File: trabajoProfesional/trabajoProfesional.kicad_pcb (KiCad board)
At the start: 2 copper layers, 191.6 x 115.6 mm, 130 parts

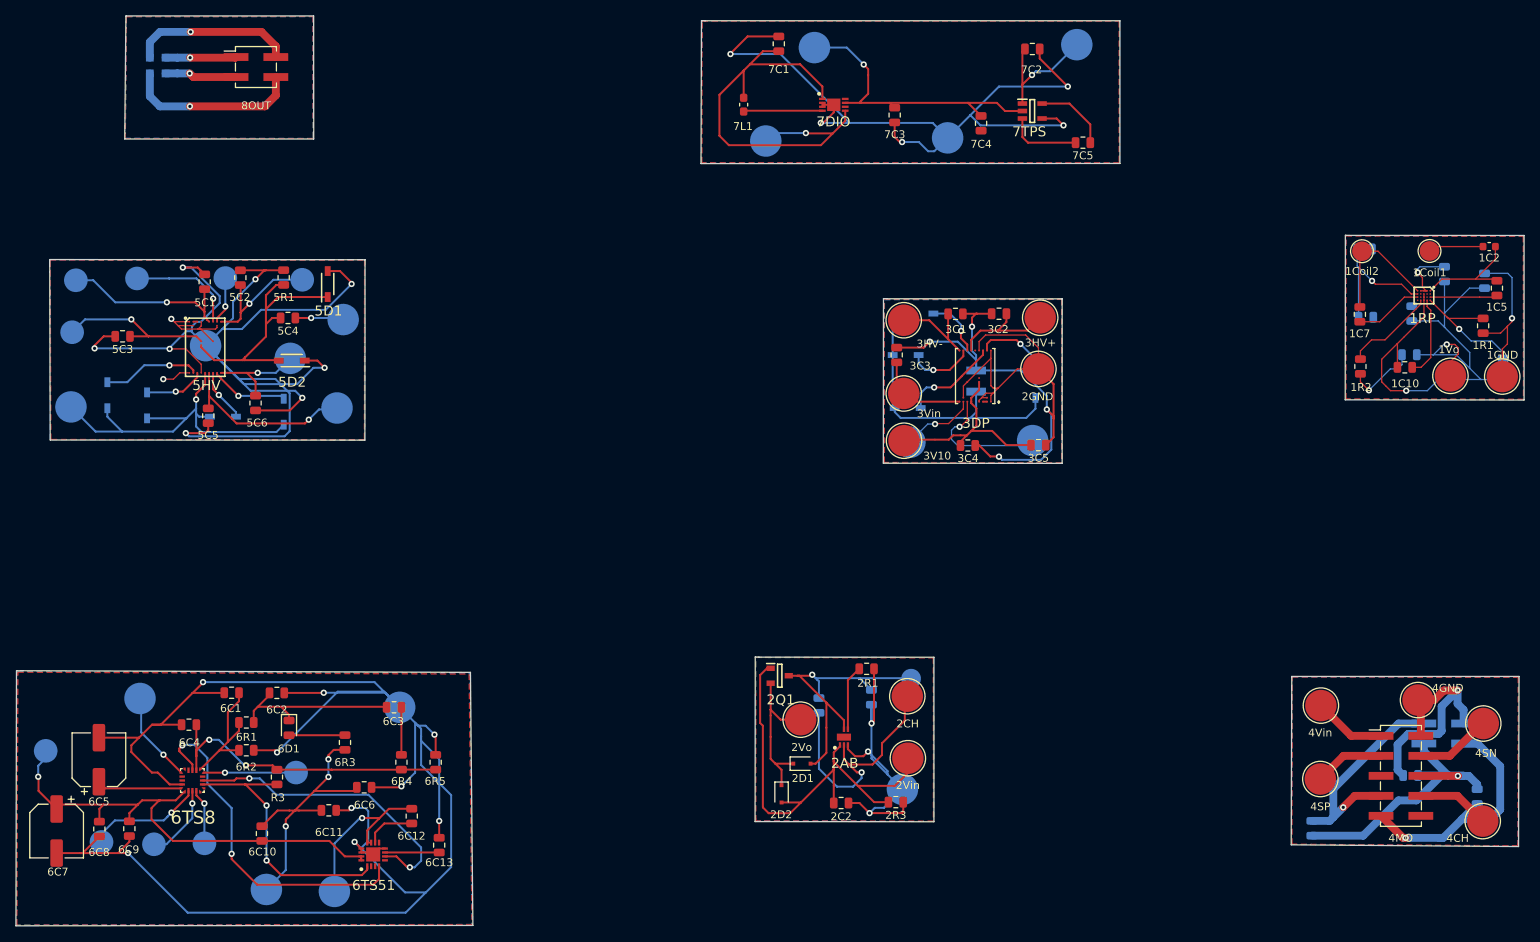
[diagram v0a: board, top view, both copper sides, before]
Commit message: se unifica todo
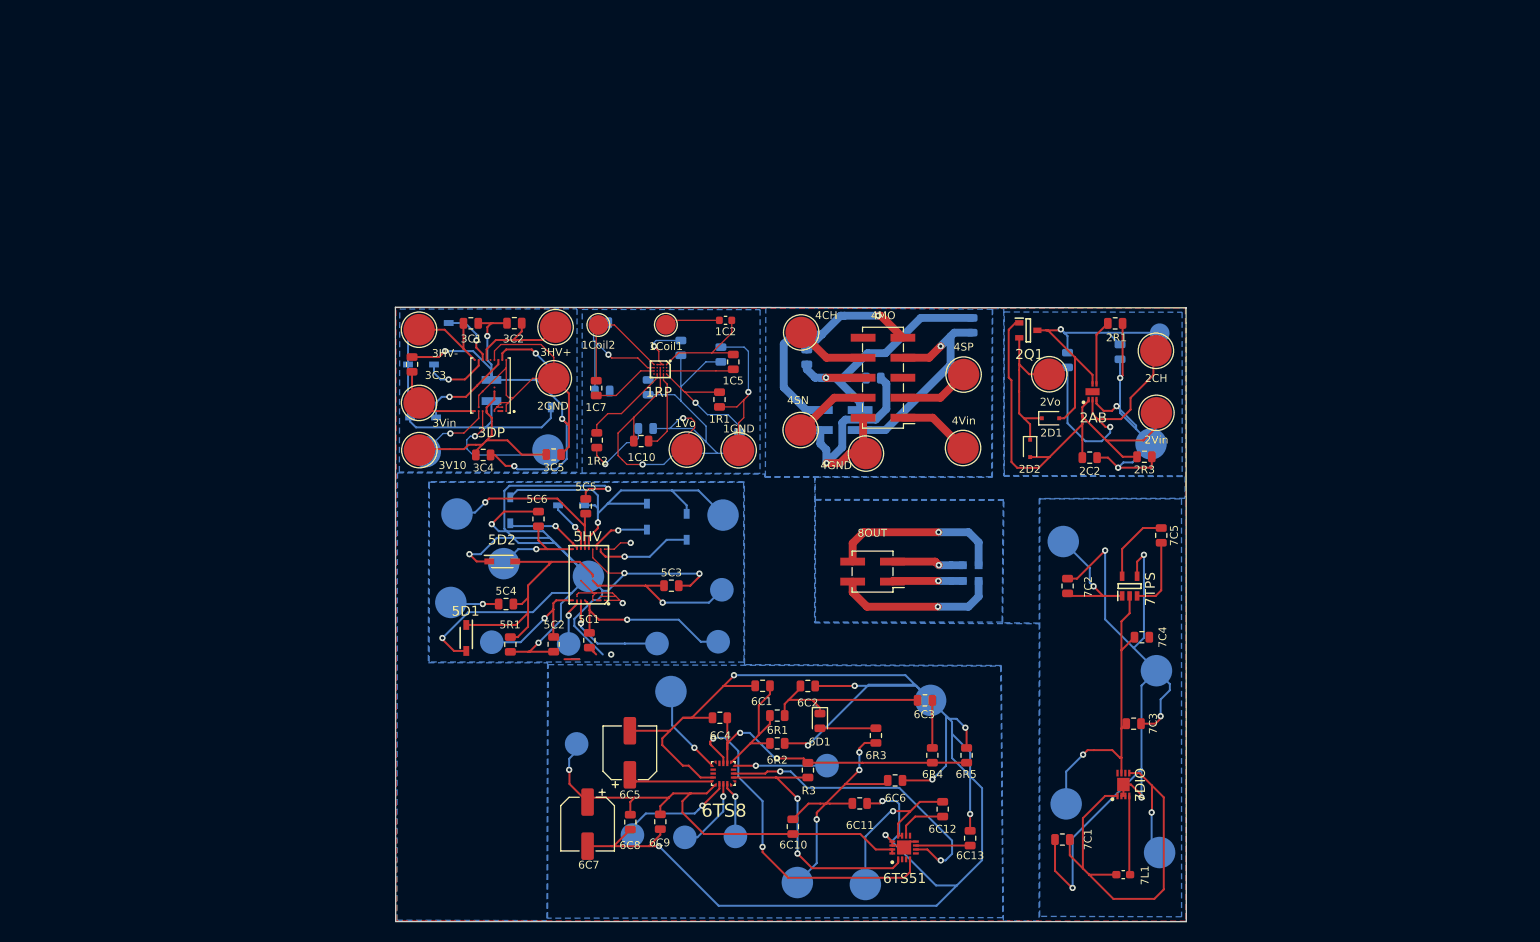
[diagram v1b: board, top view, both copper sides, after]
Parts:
- moved 8MS 121.8 mm to (148.3, 92.0), turned to 180 degrees
- moved 7L1 109.1 mm to (167.7, 130.3), turned to 0 degrees
- moved 7C1 107.3 mm to (159.9, 125.9), turned to 0 degrees
- moved 4CH 106.5 mm to (126.8, 61.5), turned to 180 degrees
- moved 7V3.3 103.3 mm to (172.3, 127.5), turned to 90 degrees
- moved 4R1 101.9 mm to (127.5, 64.6), turned to 90 degrees
- moved 7V5 101.3 mm to (160.4, 121.3), turned to 90 degrees
- moved 8OUT 101.2 mm to (135.8, 91.8), turned to 180 degrees
- moved 1C4 97.5 mm to (116.6, 64.2)
- moved 1GND 97.5 mm to (118.8, 76.4)
- moved 1C1 97.5 mm to (101.3, 60.2)
- moved 1C3 97.5 mm to (111.5, 63.4)
- moved 1C5 97.5 mm to (118.1, 65.2)
- moved 1C7 97.5 mm to (100.7, 68.5)
- moved 1C8 97.5 mm to (107.3, 68.4)
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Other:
- board size 191.6 x 115.6 mm -> 100.5 x 78.1 mm
